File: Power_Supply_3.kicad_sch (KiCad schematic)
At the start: 12 parts

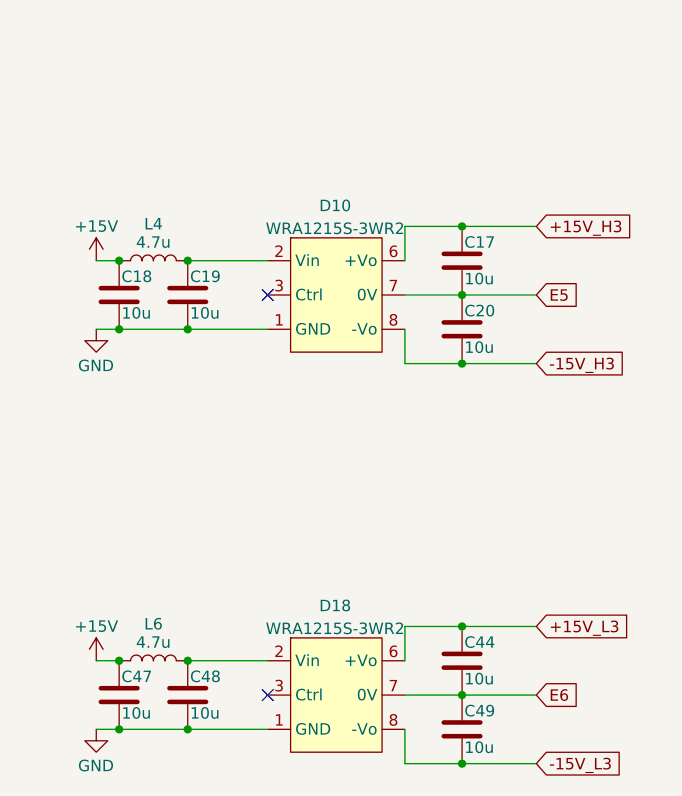
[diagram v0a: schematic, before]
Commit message: VER2.2: все изменения в списке изменений
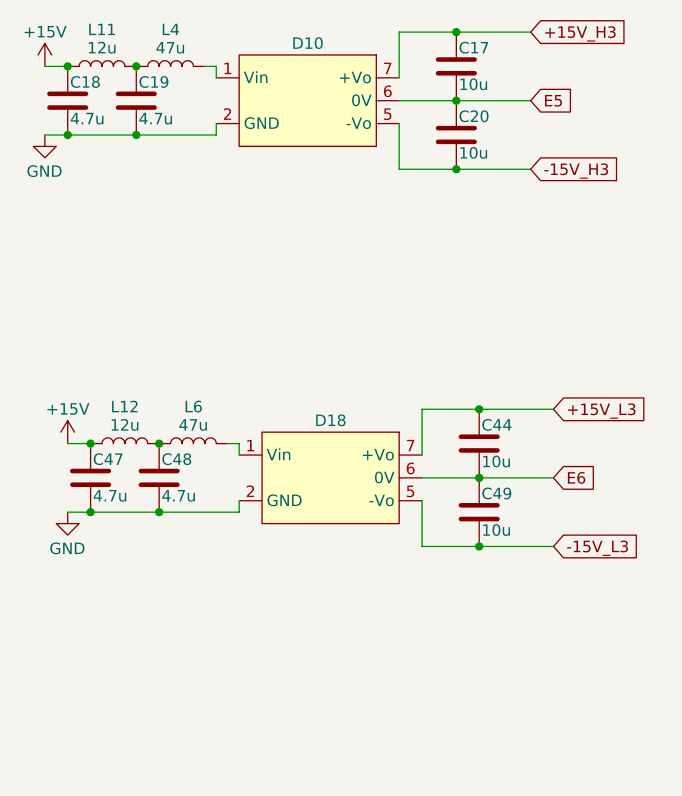
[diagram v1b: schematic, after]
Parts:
- removed D10, D18: WRA1215S-3WR2, Mornsun:WRA_S-3WR2, symbol Morsun:WRA1215S-3WR2
- added D10, D18: ~, DCDC_My:QA, symbol DCDC_My:QA1
- added L11, L12: 12u, Inductor_SMD:L_1210_3225Metric_Pad1.42x2.65mm_HandSolder, symbol Device:L
- C18, C19, C47, C48: value 10u -> 4.7u; footprint Capacitor_SMD:C_1210_3225Metric_Pad1.33x2.70mm_HandSolder -> Capacitor_SMD:C_1206_3216Metric_Pad1.33x1.80mm_HandSolder
- L4, L6: value 4.7u -> 47u; Product Name (none) -> LQH43CN470K03L
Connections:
- net +15V: now also L11.1, L12.1; no longer L4.1, L6.1
- net +15V_H3: now also D10.7 (+Vo)
- net +15V_L3: now also D18.7 (+Vo)
- net -15V_H3: now also D10.5 (-Vo)
- net -15V_L3: now also D18.5 (-Vo)
- net E5: now also D10.6 (0V)
- net E6: now also D18.6 (0V)
- net GND: now also D10.2 (GND), D18.2 (GND)
- net at C19.1: now also L4.1, L11.2; no longer L4.2
- net at C48.1: now also L6.1, L12.2; no longer L6.2
- new net: D10.1 (Vin), L4.2
- new net: D18.1 (Vin), L6.2
- no-connect marks 2 -> 0
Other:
- moved on the sheet: C17, C18, C19, C20, C44, C47, C48, C49, L4, L6
